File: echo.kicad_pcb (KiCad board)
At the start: 2 copper layers, 99 x 74 mm, 115 parts, among them J1 USB4215-03-A, J10 D-SUB 9 Male, J11 MDC-036, J2 D-SUB 9 Male, J3 MDC-036, J4 D-SUB 15 Female, J5 0475710001, J6 104031-0811, J7 PJ-320D, J8 676430910, J9 PJ-320D, Q1 BSS138, Q2 BSS138, Q3 AO3400A, Q4 AO3400A, Q5 AO3400A, Q6 AO3400A, U1 SN74CBT3257CDR, U2 CH340C, U3 NCP1117 3.3, U4 USBLC6-2SC6, U5 ESP32-WROVER-E, U6 USBLC6-2SC6, U7 W25Q128JVSIQ, U8 RP2040, Y1 12 MHz

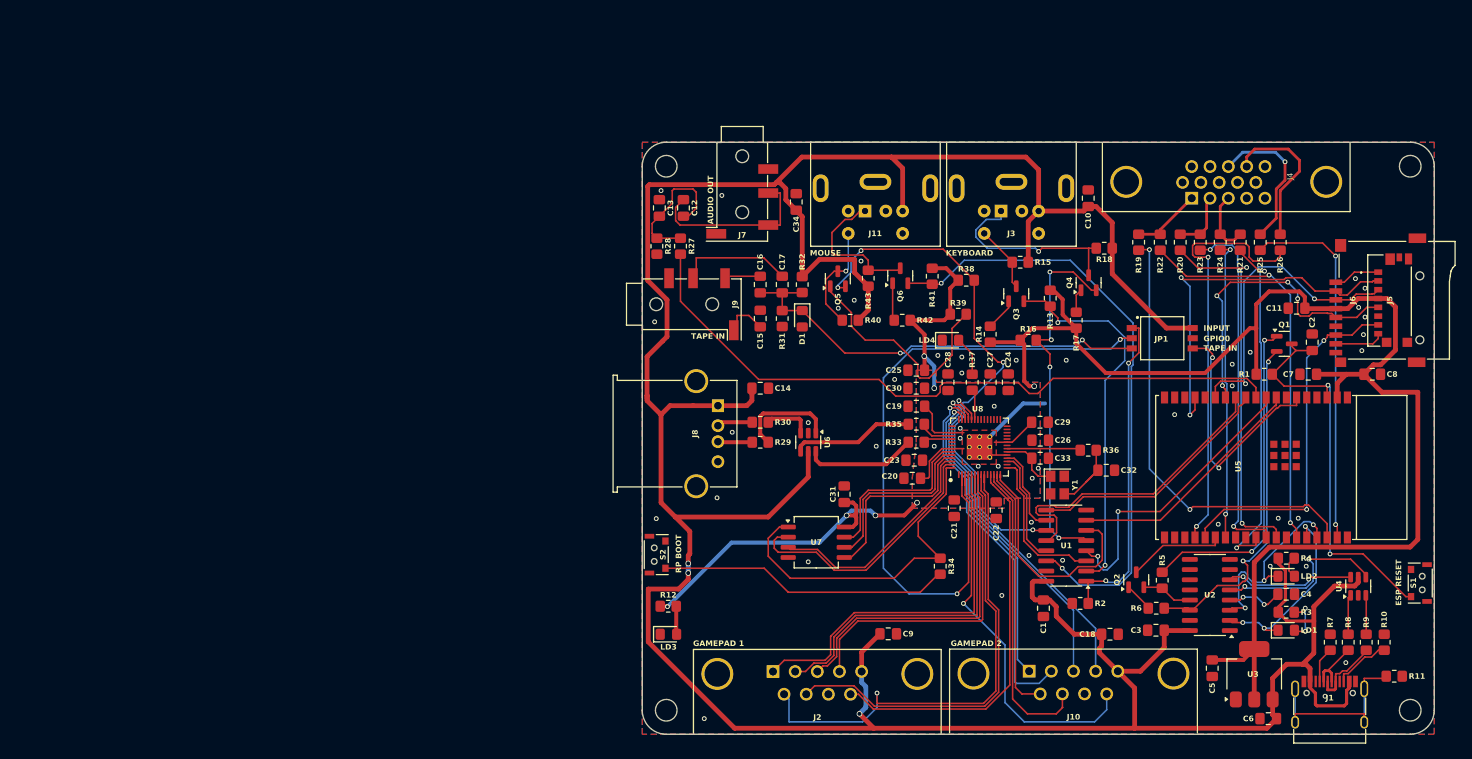
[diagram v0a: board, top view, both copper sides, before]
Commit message: Minor fixes
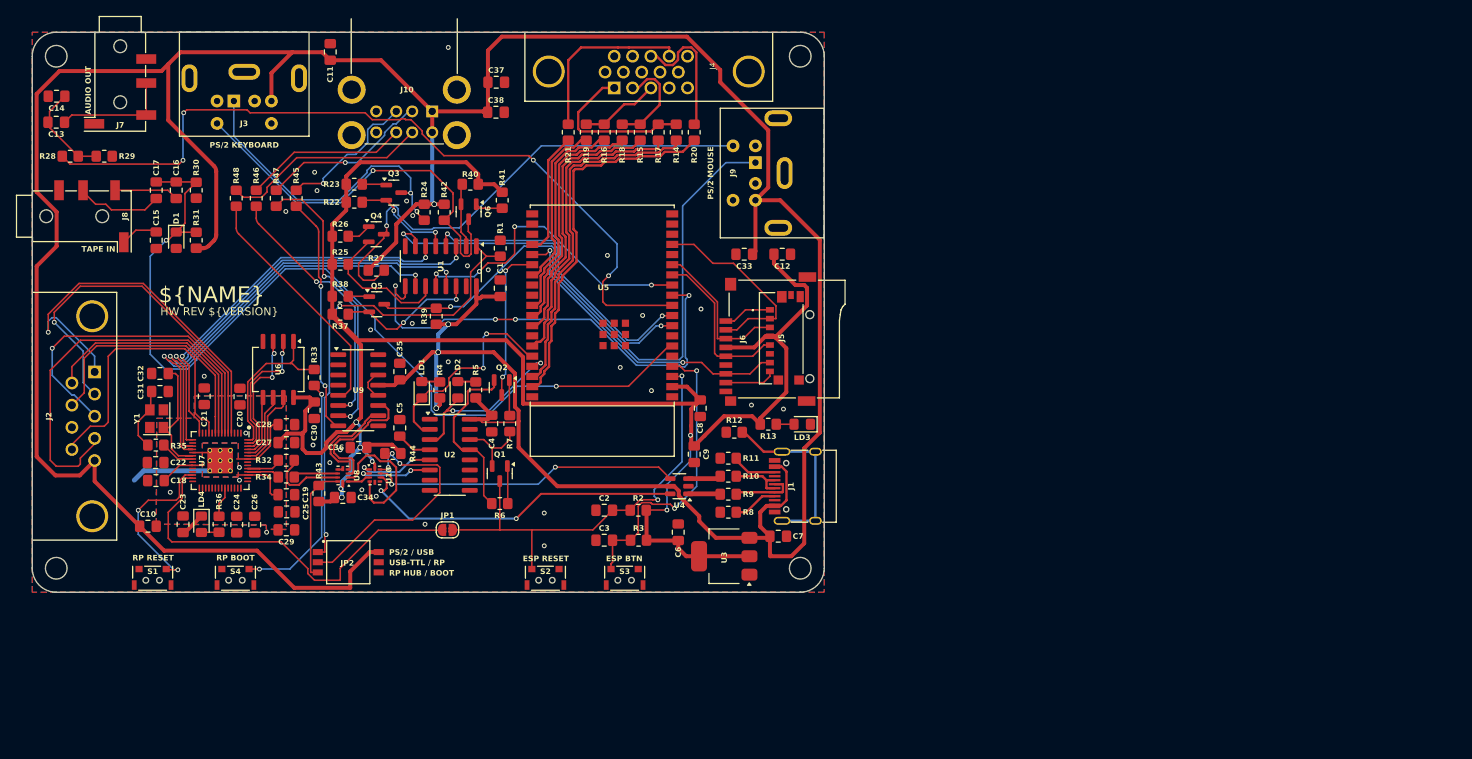
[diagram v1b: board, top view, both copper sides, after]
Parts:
- removed J11: MDC-036, FRANK:MiniDIN (6 Pin, female)
- added C35: 4.7u, FRANK:Capacitor (0805), F.Cu at (120.9, 91.4)
- added C36: 100n, FRANK:Capacitor (0805), F.Cu at (115.8, 100.9)
- added C37: 10u, FRANK:Capacitor (0805), F.Cu at (133.0, 55.2)
- added C38: 10u, FRANK:Capacitor (0805), F.Cu at (133.0, 59.0)
- added JP2: Main Jumpers, FRANK:SW_DS05-127-2-03BK-SMT-TR, F.Cu at (114.5, 115.2)
- added R44: 10K, FRANK:Resistor (0805), F.Cu at (120.1, 101.7)
- added R45: 22R, FRANK:Resistor (0805), F.Cu at (108.0, 69.8)
- added R46: 22R, FRANK:Resistor (0805), F.Cu at (103.0, 69.8)
- added R47: 22R, FRANK:Resistor (0805), F.Cu at (105.5, 69.8)
- added R48: 22R, FRANK:Resistor (0805), F.Cu at (100.5, 69.8)
- added S3: ESP Ctrl, FRANK:TACT-SIDE-4623, F.Cu at (149.1, 117.5)
- added S4: RP Boot, FRANK:TACT-SIDE-4623, F.Cu at (100.4, 117.5)
- added U10: TS3USB221RSER, FRANK:UQFN-10, F.Cu at (117.8, 104.4)
- added U9: MW7211A, FRANK:SOP-16, F.Cu at (115.8, 93.8)
- C12, C5: value 10u -> 100n
- C13: value 33n -> 10u
- C14: value 10u -> 33n
- C28, C3: value 100n -> 1u
- C30: value 1u -> 100n
- C31: value 100n -> 15p
- C33: value 15p -> 100n
- C8: value 100n -> 10u
- J10: value D-SUB 9 Male -> SS-52100-004; footprint FRANK:D-SUB (9 pin, male, top mount) -> FRANK:USB Type A (stacked)
- J8: value 676430910 -> PJ-320D; footprint FRANK:USB Type A (single) -> FRANK:Jack (3.5mm, PJ-320D)
- J9: value PJ-320D -> MDC-036; footprint FRANK:Jack (3.5mm, PJ-320D) -> FRANK:MiniDIN (6 Pin, female)
- JP1: value Main Jumpers -> ESP-RP RST; footprint FRANK:SW_DS05-127-2-03BK-SMT-TR -> FRANK:Jumper (solder)
- LD1: value TX -> Orange (TX)
- LD2: value RX -> Orange (RX)
- LD3: value Power -> Green (Power)
- LD4: value Blue -> Blue (GPIO25)
- R10: value 5.1K -> 22R
- R11: value 1M -> 5.1K
- R12: value 1K -> 1M
- R13, R18: value 22K -> 1K
- R14: value 4.7K -> 330R
- R15, R16: value 22K -> 330R
- R17: value 4.7K -> 1K
- R19: value 330R -> 1K
- R20, R21: value 330R -> 100R
- R22, R24, R37: value 1K -> 22K
- R23: value 1K -> 4.7K
- R25, R27: value 100R -> 22K
- R26: value 100R -> 4.7K
- R28: value 150R -> 100R
- R29: value 22R -> 150R
- R3: value 1.5K -> 10K
- R30: value 22R -> 10K
- R32: value 10K -> 27R
- R33, R35: value 27R -> 1K
- R34: value 1K -> 27R
- R38, R41: value 22K -> 4.7K
- R39, R42: value 4.7K -> 22K
- R43: value 22K -> 10K
- R5: value 2.2K -> 1.5K
- R7: value 5.1K -> 2.2K
- R8: value 22R -> 5.1K
- S1: value Reset -> RP Reset
- S2: value Boot -> ESP Reset
- U6: value USBLC6-2SC6 -> W25Q128JVSIQ; footprint FRANK:SOT-23-6 -> FRANK:SOIC-8
- U7: value W25Q128JVSIQ -> RP2040; footprint FRANK:SOIC-8 -> FRANK:QFN 56
- U8: value RP2040 -> TS3USB221RSER; footprint FRANK:QFN 56 -> FRANK:UQFN-10
- moved S1 158.7 mm to (90.0, 117.5), turned to 180 degrees
- moved C11 125.0 mm to (112.2, 51.5), turned to 90 degrees
- moved C10 124.5 mm to (89.5, 110.8), turned to 0 degrees
- moved C18 120.8 mm to (90.5, 105.0), turned to 180 degrees
- moved C32 118.9 mm to (91.0, 91.7), turned to 180 degrees
- moved R26 117.5 mm to (113.5, 74.5), turned to 0 degrees
- moved R25 115.0 mm to (113.5, 78.0), turned to 0 degrees
- moved Y1 112.9 mm to (90.5, 97.3), turned to 90 degrees
- moved LD1 112.2 mm to (123.7, 93.7), turned to 90 degrees
- moved R36 109.0 mm to (98.3, 110.5), turned to 90 degrees
- moved R4 107.9 mm to (125.9, 93.7), turned to -90 degrees
- moved LD2 106.2 mm to (128.2, 93.7), turned to 90 degrees
- moved R7 106.1 mm to (134.7, 97.9)
- moved R23 106.0 mm to (115.2, 68.0), turned to 0 degrees
- moved C5 105.9 mm to (120.9, 98.5), turned to 90 degrees
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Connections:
- net /SENSOR_VN renamed /ESP_IO39
- C11 pad 1: GND -> VBUS
- C11 pad 2: +3V3 -> GND
- C12 pad 1: /Audio Out/A_OUT -> GND
- C12 pad 2: Net-(C12-Pad2) -> +3V3
- C13 pad 1: GND -> /Audio Out/A_OUT
- C13 pad 2: Net-(C12-Pad2) -> Net-(C13-Pad2)
- C14 pad 2: VBUS -> Net-(C13-Pad2)
- C16 pad 1: /LOAD_IN -> /ESP_IO34
- C17 pad 1: /LOAD_IN -> /ESP_IO34
- C18 pad 1: VBUS -> Net-(U7-VREG_VOUT)
- C19 pad 1: Net-(U8-VREG_VOUT) -> Net-(U7-VREG_VOUT)
- C20 pad 1: Net-(U8-VREG_VOUT) -> +3V3
- C28 pad 1: +3V3 -> Net-(U7-VREG_VOUT)
- C29 pad 1: Net-(U8-VREG_VOUT) -> +3V3
- C3 pad 1: VBUS -> /ESP_IO36
- C31 pad 1: +3V3 -> Net-(C31-Pad1)
- C32 pad 1: Net-(C32-Pad1) -> /RP2040/XIN
- C33 pad 1: /RP2040/XIN -> VBUS
- C34 pad 1: VBUS -> GND
- C34 pad 2: GND -> +3V3
- C4 pad 1: Net-(U2-3V) -> VBUS
- C5 pad 1: +3V3 -> Net-(U2-3V)
- C6 pad 1: VBUS -> +3V3
- C7 pad 1: +3V3 -> VBUS
- C9 pad 1: VBUS -> +3V3
- D1 pad 1: /LOAD_IN -> /ESP_IO34
- J10 pad 1: /GPIO29 -> VBUS
- J10 pad 2: /GPIO28 -> Net-(J10-D1-)
- J10 pad 3: /GPIO27 -> Net-(J10-D1+)
- J10 pad 4: /GPIO26 -> GND
- J10 pad 6: /GPIO10 -> Net-(J10-D2-)
- J10 pad 7: /GPIO9 -> Net-(J10-D2+)
- J10 pad 9: /GPIO1 -> GND
- J3 pad 1: /PS2 KB/DATA -> /KB_DATA
- J3 pad 5: /PS2 KB/CLK -> /KB_CLK
- JP1 pad 1: /SN74_S -> /GPIO16
- JP1 pad 2: /GPIO0 -> /ESP_EN
- Q3 pad 2: /KB_CLK_3V -> /KB_DATA_3V
- Q3 pad 3: /PS2 KB/CLK -> /KB_DATA
- Q4 pad 2: /KB_DATA_3V -> /MS_CLK_3V
- Q4 pad 3: /PS2 KB/DATA -> /MS_CLK
- Q5 pad 2: /MS_CLK_3V -> /MS_DATA_3V
- Q5 pad 3: /PS2 MS/CLK -> /MS_DATA
- Q6 pad 2: /MS_DATA_3V -> /KB_CLK_3V
- Q6 pad 3: /PS2 MS/DATA -> /KB_CLK
- R1 pad 1: /ESP_EN -> GND
- R1 pad 2: +3V3 -> /SN74_S
- R10 pad 1: GND -> Net-(R10-Pad1)
- R10 pad 2: Net-(J1-CC2) -> Net-(J1-DP1)
- R11 pad 1: Net-(J1-SHIELD) -> GND
- R11 pad 2: GND -> Net-(J1-CC2)
- R12 pad 1: Net-(LD3-A) -> Net-(J1-SHIELD)
- R12 pad 2: +3V3 -> GND
- R13 pad 1: +3V3 -> Net-(LD3-A)
- R13 pad 2: /KB_CLK_3V -> +3V3
- R14 pad 1: +3V3 -> /ESP_IO22
- R14 pad 2: Net-(Q3-G) -> Net-(J4-Pad1)
- R15 pad 1: VBUS -> /ESP_IO19
- R15 pad 2: /PS2 KB/CLK -> Net-(J4-Pad2)
- R16 pad 1: +3V3 -> /ESP_IO5
- R16 pad 2: /KB_DATA_3V -> Net-(J4-Pad3)
- R17 pad 1: +3V3 -> /ESP_IO21
- R17 pad 2: Net-(Q4-G) -> Net-(J4-Pad1)
- R18 pad 1: VBUS -> /ESP_IO18
- R18 pad 2: /PS2 KB/DATA -> Net-(J4-Pad2)
- R19 pad 1: /ESP_IO22 -> /ESP_IO4
- R19 pad 2: Net-(J4-Pad1) -> Net-(J4-Pad3)
- R2 pad 1: GND -> /ESP_EN
- R2 pad 2: /SN74_S -> +3V3
- R20 pad 1: /ESP_IO19 -> Net-(J4-Pad13)
- R20 pad 2: Net-(J4-Pad2) -> /ESP_IO23
- R21 pad 1: /ESP_IO5 -> Net-(J4-Pad14)
- R21 pad 2: Net-(J4-Pad3) -> /ESP_IO15
- R22 pad 1: /ESP_IO21 -> +3V3
- R22 pad 2: Net-(J4-Pad1) -> /KB_DATA_3V
- R23 pad 1: /ESP_IO18 -> +3V3
- R23 pad 2: Net-(J4-Pad2) -> Net-(Q3-G)
- R24 pad 1: /ESP_IO4 -> VBUS
- R24 pad 2: Net-(J4-Pad3) -> /KB_DATA
- R25 pad 1: Net-(J4-Pad13) -> +3V3
- R25 pad 2: /ESP_IO23 -> /MS_CLK_3V
- R26 pad 1: Net-(J4-Pad14) -> +3V3
- R26 pad 2: /ESP_IO15 -> Net-(Q4-G)
- R27 pad 1: /ESP_IO25 -> VBUS
- R27 pad 2: Net-(C12-Pad2) -> /MS_CLK
- R28 pad 1: GND -> /ESP_IO25
- R28 pad 2: Net-(C12-Pad2) -> Net-(C13-Pad2)
- R29 pad 1: Net-(R29-Pad1) -> GND
- R29 pad 2: Net-(J8-D+) -> Net-(C13-Pad2)
- R3 pad 1: Net-(LD1-A) -> /ESP_IO36
- R3 pad 2: VBUS -> +3V3
- R30 pad 1: Net-(R30-Pad1) -> /ESP_IO34
- R30 pad 2: Net-(J8-D-) -> GND
- R31 pad 1: /LOAD_IN -> /ESP_IO34
- R31 pad 2: GND -> VBUS
- R32 pad 1: /LOAD_IN -> /RP_D+
- R32 pad 2: VBUS -> Net-(U7-USB_DP)
- R33 pad 1: /RP_D+ -> /RP2040/QSPI_SS
- R33 pad 2: Net-(U8-USB_DP) -> Net-(R33-Pad2)
- R34 pad 1: /RP2040/QSPI_SS -> /RP_D-
- R34 pad 2: Net-(R34-Pad2) -> Net-(U7-USB_DM)
- R35 pad 1: /RP_D- -> /RP2040/XOUT
- R35 pad 2: Net-(U8-USB_DM) -> Net-(C31-Pad1)
- R36 pad 1: /RP2040/XOUT -> Net-(LD4-A)
- R36 pad 2: Net-(C32-Pad1) -> /RP2040/GPIO25
- R37 pad 1: Net-(LD4-A) -> +3V3
- R37 pad 2: /RP2040/GPIO25 -> /MS_DATA_3V
- R38 pad 2: /MS_CLK_3V -> Net-(Q5-G)
- R39 pad 1: +3V3 -> VBUS
- R39 pad 2: Net-(Q5-G) -> /MS_DATA
- R4 pad 1: VBUS -> Net-(LD1-A)
- R4 pad 2: Net-(LD2-A) -> VBUS
- R40 pad 1: VBUS -> +3V3
- R40 pad 2: /PS2 MS/CLK -> /KB_CLK_3V
- R41 pad 2: /MS_DATA_3V -> Net-(Q6-G)
- R42 pad 1: +3V3 -> VBUS
- R42 pad 2: Net-(Q6-G) -> /KB_CLK
- R43 pad 1: VBUS -> +3V3
- R43 pad 2: /PS2 MS/DATA -> /UMSW2
- R5 pad 1: Net-(Q1-B) -> VBUS
- R5 pad 2: Net-(Q2-E) -> Net-(LD2-A)
- R6 pad 1: Net-(Q2-B) -> Net-(Q1-B)
- R6 pad 2: Net-(Q1-E) -> Net-(Q2-E)
- R7 pad 1: GND -> Net-(Q2-B)
- R7 pad 2: Net-(J1-CC1) -> Net-(Q1-E)
- R8 pad 1: Net-(R8-Pad1) -> GND
- R8 pad 2: Net-(J1-DN1) -> Net-(J1-CC1)
- R9 pad 2: Net-(J1-DP1) -> Net-(J1-DN1)
- S1 pad 1: GND -> /RUN
- S1 pad 2: /ESP_EN -> GND
- S2 pad 1: Net-(R34-Pad2) -> GND
- S2 pad 2: GND -> /ESP_EN
- U2 pad 5: /PW_D+ -> /UTC_D+
- U2 pad 6: /PW_D- -> /UTC_D-
- U4 pad 1: Net-(R8-Pad1) -> Net-(R9-Pad1)
- U4 pad 3: Net-(R9-Pad1) -> Net-(R10-Pad1)
- U5 pad 4: /SENSOR_VP -> /ESP_IO36
- U6 pad 1: Net-(R29-Pad1) -> /RP2040/QSPI_SS
- U6 pad 2: GND -> /RP2040/QSPI_SD1
- U6 pad 3: Net-(R30-Pad1) -> /RP2040/QSPI_SD2
- U6 pad 4: /RP_D- -> GND
- U6 pad 5: VBUS -> /RP2040/QSPI_SD0
- U6 pad 6: /RP_D+ -> /RP2040/QSPI_SCLK
- U7 pad 1: /RP2040/QSPI_SS -> +3V3
- U7 pad 2: /RP2040/QSPI_SD1 -> /GPIO0
- U7 pad 3: /RP2040/QSPI_SD2 -> /GPIO1
- U7 pad 4: GND -> /GPIO2
- U7 pad 5: /RP2040/QSPI_SD0 -> /GPIO3
- U7 pad 6: /RP2040/QSPI_SCLK -> /GPIO4
- U7 pad 7: /RP2040/QSPI_SD3 -> /GPIO5
- U7 pad 8: +3V3 -> /GPIO6
- U8 pad 1: +3V3 -> /MP1_D+
- U8 pad 2: /GPIO0 -> /MP1_D-
- U8 pad 3: /GPIO1 -> /HUB_D+
- U8 pad 4: /GPIO2 -> /HUB_D-
- U8 pad 5: /GPIO3 -> GND
- U8 pad 6: /GPIO4 -> GND
- U8 pad 7: /GPIO5 -> /RP_D-
- U8 pad 8: /GPIO6 -> /RP_D+
- U8 pad 9: /GPIO7 -> /UMSW2
- Y1 pad 3: Net-(C32-Pad1) -> Net-(C31-Pad1)
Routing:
- net /GPIO0: track 84.6 -> 0.00 mm, vias 2 -> 0
- net /ESP_IO34: track 31.6 -> 116.1 mm
- net /MS_DATA: track 0.00 -> 79.0 mm, vias 0 -> 1
- net /MS_CLK: track 0.00 -> 63.0 mm, vias 0 -> 1
- net /MS_DATA_3V: track 76.4 -> 17.7 mm
- net /LOAD_IN: track 54.4 -> 0.00 mm, vias 2 -> 0
- net /KB_CLK: track 0.00 -> 51.3 mm, vias 0 -> 1
- net /GPIO16: track 0.00 -> 49.5 mm
- net /MS_CLK_3V: track 66.8 -> 17.8 mm, vias 4 -> 0
- net /GPIO1: track 49.0 -> 0.00 mm, vias 1 -> 0
- net /GPIO28: track 46.4 -> 0.00 mm, vias 1 -> 0
- net /GPIO26: track 45.2 -> 0.00 mm, vias 1 -> 0
- net /GPIO27: track 43.9 -> 0.00 mm, vias 1 -> 0
- net /GPIO15: track 11.0 -> 53.7 mm, vias 0 -> 2
- net /GPIO14: track 14.2 -> 56.2 mm, vias 0 -> 2
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- added copper zone on B.Cu, net Net-(U7-VREG_VOUT)
- added copper zone on F.Cu, net Net-(U7-VREG_VOUT)
- removed copper zone on F.Cu, net Net-(U8-VREG_VOUT)
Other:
- board size 99 x 74 mm -> 99 x 70 mm
- board text added: "ESP BTN"
- board text added: "HW REV ${VERSION}"
- board text added: "PS/2 / USB"
- board text added: "PS/2 KEYBOARD"
- board text added: "PS/2 MOUSE"
- board text added: "RP HUB / BOOT"
- board text added: "RP RESET"
- board text added: "USB-TTL / RP"
- board text removed: "${VERSION}"
- board text removed: "GAMEPAD 1"
- board text removed: "GAMEPAD 2"
- board text removed: "GPIO0"
- board text removed: "INPUT"
- board text removed: "KEYBOARD"
- board text removed: "MOUSE"
